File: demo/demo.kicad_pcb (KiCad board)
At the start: 4 copper layers, 30 x 30 mm, 7 parts, among them J1 USB_C_Receptacle_PowerOnly_6P, SW1 SW_Push, U1 ATtiny85-20P

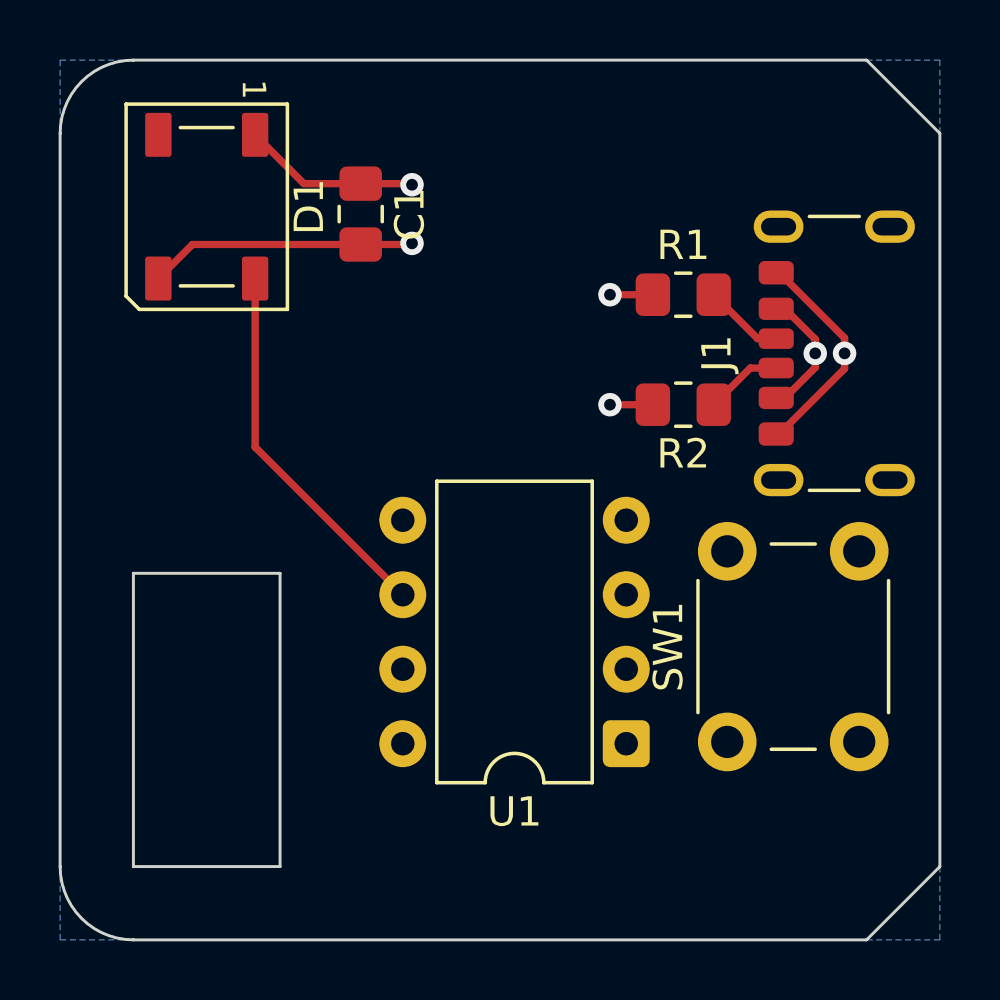
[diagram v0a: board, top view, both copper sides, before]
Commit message: demo work
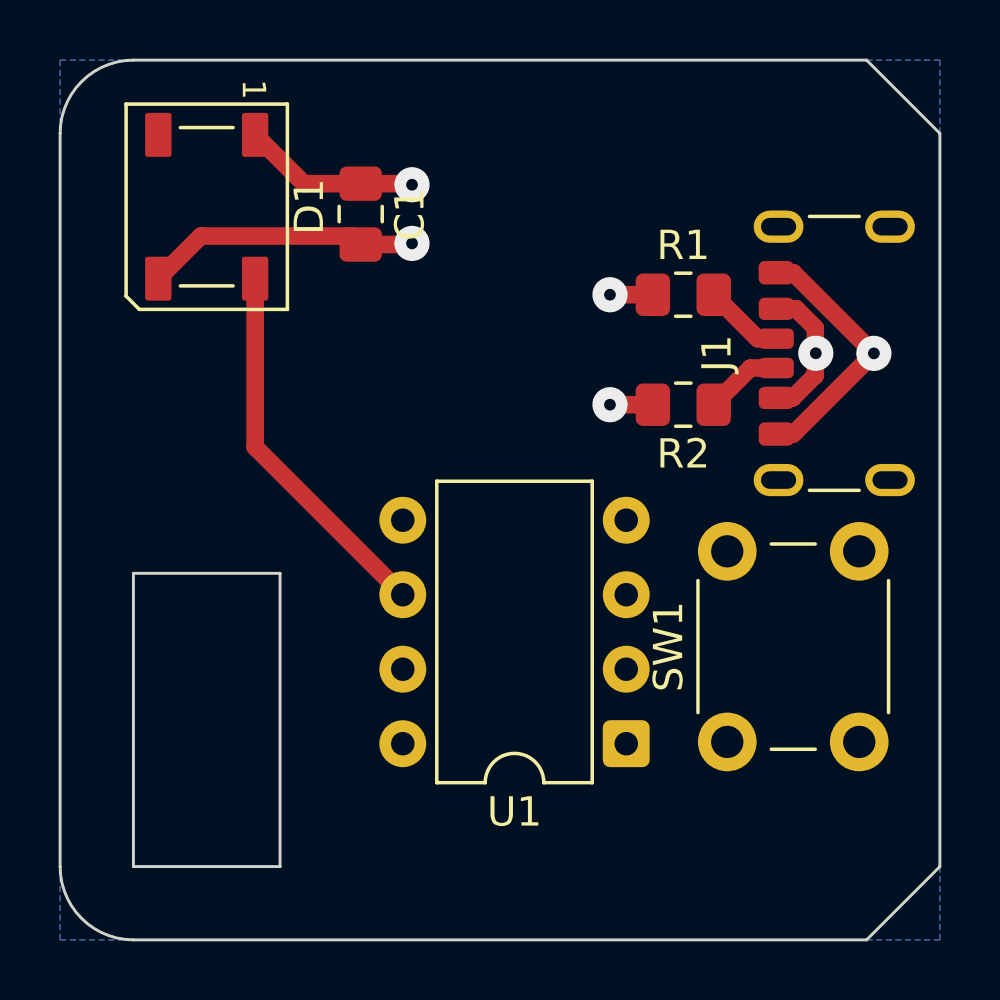
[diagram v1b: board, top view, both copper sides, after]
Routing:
- net GND: track 19.6 -> 21.2 mm
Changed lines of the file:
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@@
 	)
 	(segment
-		(start 149.25 82.5)
-		(end 149.25 81.975002)
-		(width 0.25)
-		(layer "F.Cu")
-		(net 1)
-	)
-	(segment
-		(start 149.25 82.5)
-		(end 149.25 83.024998)
-		(width 0.25)
-		(layer "F.Cu")
-		(net 1)
-	)
-	(segment
-		(start 147.024998 79.75)
+		(start 147.5 85.25)
+		(end 146.92 85.25)
+		(width 0.6)
+		(layer "F.Cu")
+		(net 1)
+	)
+	(segment
+		(start 147.5 79.75)
 		(end 146.92 79.75)
-		(width 0.25)
+		(width 0.6)
 		(layer "F.Cu")
 		(net 1)
@@
 		(start 142.7125 84.25)
 		(end 141.25 84.25)
-		(width 0.25)
-		(layer "F.Cu")
-		(net 1)
-	)
-	(segment
-		(start 132.75 78.7875)
-		(end 127.0125 78.7875)
-		(width 0.25)
-		(layer "F.Cu")
-		(net 1)
-	)
-	(segment
-		(start 149.25 83.024998)
-		(end 147.024998 85.25)
-		(width 0.25)
-		(layer "F.Cu")
-		(net 1)
-	)
-	(segment
-		(start 149.25 81.975002)
-		(end 147.024998 79.75)
-		(width 0.25)
+		(width 0.6)
 		(layer "F.Cu")
 		(net 1)
@@
 		(start 142.7125 80.5)
 		(end 141.25 80.5)
-		(width 0.25)
-		(layer "F.Cu")
-		(net 1)
-	)
-	(segment
-		(start 127.0125 78.7875)
-		(end 125.85 79.95)
-		(width 0.25)
-		(layer "F.Cu")
-		(net 1)
-	)
-	(segment
-		(start 147.024998 85.25)
-		(end 146.92 85.25)
-		(width 0.25)
+		(width 0.6)
+		(layer "F.Cu")
+		(net 1)
+	)
+	(segment
+		(start 132.4625 78.5)
+		(end 127.3 78.5)
+		(width 0.6)
 		(layer "F.Cu")
 		(net 1)
@@
 		(start 132.75 78.7875)
 		(end 134.4625 78.7875)
-		(width 0.25)
+		(width 0.6)
+		(layer "F.Cu")
+		(net 1)
+	)
+	(segment
+		(start 127.3 78.5)
+		(end 125.85 79.95)
+		(width 0.6)
 		(layer "F.Cu")
 		(net 1)
@@
 		(start 134.4625 78.7875)
 		(end 134.5 78.75)
-		(width 0.25)
+		(width 0.6)
+		(layer "F.Cu")
+		(net 1)
+	)
+	(segment
+		(start 132.75 78.7875)
+		(end 132.4625 78.5)
+		(width 0.6)
+		(layer "F.Cu")
+		(net 1)
+	)
+	(segment
+		(start 150.25 82.5)
+		(end 147.5 85.25)
+		(width 0.6)
+		(layer "F.Cu")
+		(net 1)
+	)
+	(segment
+		(start 150.25 82.5)
+		(end 147.5 79.75)
+		(width 0.6)
 		(layer "F.Cu")
 		(net 1)
@@
 	(via
 		(at 141.25 80.5)
-		(size 0.8)
+		(size 1.2)
 		(drill 0.4)
 		(layers "F.Cu" "B.Cu")
@@
 	(via
 		(at 134.5 78.75)
-		(size 0.8)
-		(drill 0.4)
-		(layers "F.Cu" "B.Cu")
-		(net 1)
-	)
-	(via
-		(at 149.25 82.5)
-		(size 0.8)
+		(size 1.2)
+		(drill 0.4)
+		(layers "F.Cu" "B.Cu")
+		(net 1)
+	)
+	(via
+		(at 150.25 82.5)
+		(size 1.2)
 		(drill 0.4)
 		(layers "F.Cu" "B.Cu")
@@
 	(via
 		(at 141.25 84.25)
-		(size 0.8)
-		(drill 0.4)
-		(layers "F.Cu" "B.Cu")
-		(net 1)
-	)
-	(segment
-		(start 148.25 82.01663)
-		(end 148.25 82.5)
-		(width 0.25)
-		(layer "F.Cu")
-		(net 2)
-	)
-	(segment
-		(start 146.92 80.98)
-		(end 147.21337 80.98)
-		(width 0.25)
+		(size 1.2)
+		(drill 0.4)
+		(layers "F.Cu" "B.Cu")
+		(net 1)
+	)
+	(segment
+		(start 148.25 81.632786)
+		(end 147.597214 80.98)
+		(width 0.6)
+		(layer "F.Cu")
+		(net 2)
+	)
+	(segment
+		(start 148.25 82.514659)
+		(end 148.25 83.25)
+		(width 0.6)
+		(layer "F.Cu")
+		(net 2)
+	)
+	(segment
+		(start 148.268992 82.495667)
+		(end 148.25 82.476675)
+		(width 0.6)
 		(layer "F.Cu")
 		(net 2)
@@
 		(start 130.8125 76.7125)
 		(end 129.15 75.05)
-		(width 0.25)
+		(width 0.6)
+		(layer "F.Cu")
+		(net 2)
+	)
+	(segment
+		(start 148.268992 82.495667)
+		(end 148.25 82.514659)
+		(width 0.6)
+		(layer "F.Cu")
+		(net 2)
+	)
+	(segment
+		(start 148.25 83.25)
+		(end 147.48 84.02)
+		(width 0.6)
 		(layer "F.Cu")
 		(net 2)
@@
 		(start 132.75 76.7125)
 		(end 130.8125 76.7125)
-		(width 0.25)
-		(layer "F.Cu")
-		(net 2)
-	)
-	(segment
-		(start 148.25 82.5)
-		(end 148.25 82.98337)
-		(width 0.25)
-		(layer "F.Cu")
-		(net 2)
-	)
-	(segment
-		(start 148.25 82.98337)
-		(end 147.21337 84.02)
-		(width 0.25)
-		(layer "F.Cu")
-		(net 2)
-	)
-	(segment
-		(start 147.21337 80.98)
-		(end 148.25 82.01663)
-		(width 0.25)
-		(layer "F.Cu")
-		(net 2)
-	)
-	(segment
-		(start 147.21337 84.02)
+		(width 0.6)
+		(layer "F.Cu")
+		(net 2)
+	)
+	(segment
+		(start 147.48 84.02)
 		(end 146.92 84.02)
-		(width 0.25)
+		(width 0.6)
 		(layer "F.Cu")
 		(net 2)
@@
 		(start 132.75 76.7125)
 		(end 134.4625 76.7125)
-		(width 0.25)
+		(width 0.6)
+		(layer "F.Cu")
+		(net 2)
+	)
+	(segment
+		(start 148.25 82.476675)
+		(end 148.25 81.632786)
+		(width 0.6)
+		(layer "F.Cu")
+		(net 2)
+	)
+	(segment
+		(start 147.597214 80.98)
+		(end 146.92 80.98)
+		(width 0.6)
 		(layer "F.Cu")
 		(net 2)
@@
 		(start 134.4625 76.7125)
 		(end 134.5 76.75)
-		(width 0.25)
+		(width 0.6)
 		(layer "F.Cu")
 		(net 2)
@@
 	(via
 		(at 134.5 76.75)
-		(size 0.8)
-		(drill 0.4)
-		(layers "F.Cu" "B.Cu")
-		(net 2)
-	)
-	(via
-		(at 148.25 82.5)
-		(size 0.8)
+		(size 1.2)
+		(drill 0.4)
+		(layers "F.Cu" "B.Cu")
+		(net 2)
+	)
+	(via
+		(at 148.268992 82.495667)
+		(size 1.2)
 		(drill 0.4)
 		(layers "F.Cu" "B.Cu")
@@
 		(start 129.15 85.695)
 		(end 134.185 90.73)
-		(width 0.25)
+		(width 0.6)
 		(layer "F.Cu")
 		(net 3)
@@
 		(start 129.15 79.95)
 		(end 129.15 85.695)
-		(width 0.25)
+		(width 0.6)
 		(layer "F.Cu")
 		(net 3)
@@
 		(start 146.2875 82)
 		(end 144.7875 80.5)
-		(width 0.25)
+		(width 0.6)
 		(layer "F.Cu")
 		(net 5)
@@
 		(start 146.92 82)
 		(end 146.2875 82)
-		(width 0.25)
+		(width 0.6)
 		(layer "F.Cu")
 		(net 5)
@@
 		(start 146.0375 83)
 		(end 144.7875 84.25)
-		(width 0.25)
+		(width 0.6)
 		(layer "F.Cu")
 		(net 6)
@@
 		(start 146.92 83)
 		(end 146.0375 83)
-		(width 0.25)
+		(width 0.6)
 		(layer "F.Cu")
 		(net 6)
@@
 		(fill yes
 			(mode hatch)
-			(thermal_gap 0.5)
-			(thermal_bridge_width 0.5)
-			(hatch_thickness 1)
-			(hatch_gap 1.5)
+			(thermal_gap 1)
+			(thermal_bridge_width 1)
+			(hatch_thickness 1.2)
+			(hatch_gap 2)
 			(hatch_orientation 45)
 			(hatch_border_algorithm hatch_thickness)
@@
 		(fill yes
 			(mode hatch)
-			(thermal_gap 0.5)
-			(thermal_bridge_width 0.5)
-			(hatch_thickness 1)
-			(hatch_gap 1.5)
+			(thermal_gap 1)
+			(thermal_bridge_width 1)
+			(hatch_thickness 1.2)
+			(hatch_gap 2)
 			(hatch_orientation 45)
 			(hatch_border_algorithm hatch_thickness)
